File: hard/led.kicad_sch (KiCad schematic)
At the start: 18 parts, among them J1 WS2812B

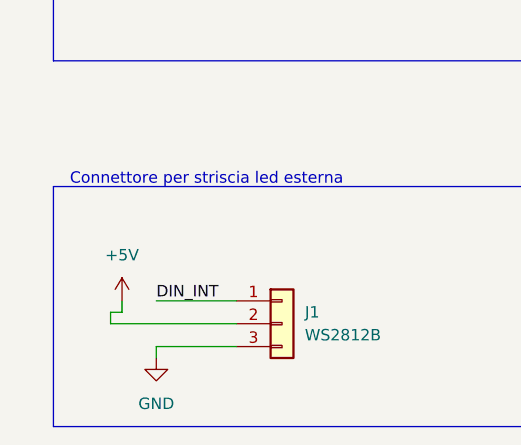
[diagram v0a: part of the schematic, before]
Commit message: update
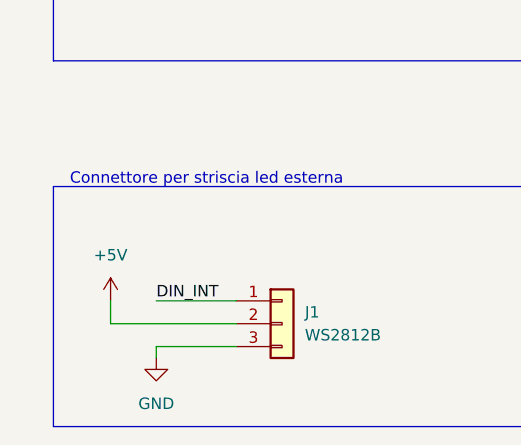
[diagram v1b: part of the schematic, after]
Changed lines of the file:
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@@
-	(wire
-		(pts
-			(xy 21.59 115.57) (xy 22.86 115.57)
-		)
-		(stroke
-			(width 0)
-			(type default)
-		)
-	)
 	(wire
 		(pts
@@
 	(wire
 		(pts
-			(xy 21.59 116.84) (xy 21.59 115.57)
-		)
-		(stroke
-			(width 0)
-			(type default)
-		)
-	)
-	(wire
-		(pts
 			(xy 129.54 39.37) (xy 129.54 50.8)
 		)
@@
 	(wire
 		(pts
-			(xy 22.86 115.57) (xy 22.86 114.3)
+			(xy 21.59 114.3) (xy 21.59 116.84)
 		)
 		(stroke
@@
 	(symbol
 		(lib_id "power:+5V")
-		(at 22.86 114.3 0)
+		(at 21.59 114.3 0)
 		(unit 1)
 		(exclude_from_sim no)
@@
 		(fields_autoplaced yes)
 		(property "Reference" "#PWR099"
-			(at 22.86 118.11 0)
+			(at 21.59 118.11 0)
 			(effects
 				(font
@@
 		)
 		(property "Value" "+5V"
-			(at 22.86 109.22 0)
+			(at 21.59 109.22 0)
 			(effects
 				(font
@@
 		)
 		(property "Footprint" ""
-			(at 22.86 114.3 0)
+			(at 21.59 114.3 0)
 			(effects
 				(font
@@
 		)
 		(property "Datasheet" ""
-			(at 22.86 114.3 0)
+			(at 21.59 114.3 0)
 			(effects
 				(font
@@
 		)
 		(property "Description" "Power symbol creates a global label with name \"+5V\""
-			(at 22.86 114.3 0)
-			(effects
-				(font
+			(at 21.59 114.3 0)
+			(effects
+				(font

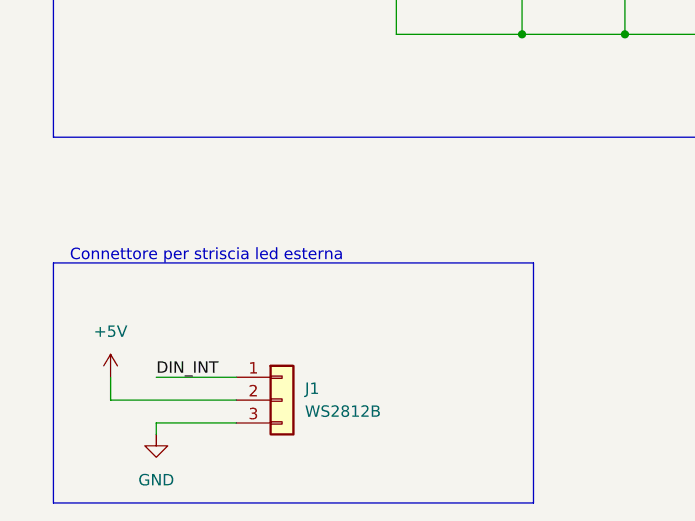
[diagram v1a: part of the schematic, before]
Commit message: update
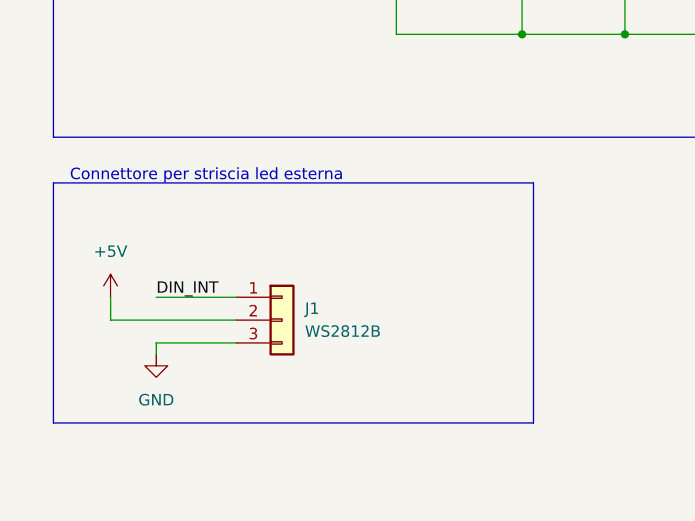
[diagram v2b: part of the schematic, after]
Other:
- title: (none) -> Moduli RGB e LED
- moved on the sheet: J1
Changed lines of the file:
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@@
 	(generator_version "9.0")
 	(paper "A4")
+	(title_block
+		(title "Moduli RGB e LED")
+	)
 	(rectangle
 		(start 15.24 17.78)
@@
 	)
 	(rectangle
-		(start 15.24 101.6)
-		(end 68.58 128.27)
+		(start 15.24 92.71)
+		(end 68.58 119.38)
 		(stroke
 			(width 0)
@@
 	(text "Connettore per striscia led esterna"
 		(exclude_from_sim no)
-		(at 32.258 100.838 0)
+		(at 32.258 91.948 0)
 		(effects
 			(font
@@
 	(wire
 		(pts
-			(xy 26.67 114.3) (xy 35.56 114.3)
+			(xy 26.67 105.41) (xy 35.56 105.41)
 		)
 		(stroke
@@
 	(wire
 		(pts
-			(xy 35.56 119.38) (xy 26.67 119.38)
+			(xy 35.56 110.49) (xy 26.67 110.49)
 		)
 		(stroke
@@
 	(wire
 		(pts
-			(xy 35.56 116.84) (xy 21.59 116.84)
+			(xy 35.56 107.95) (xy 21.59 107.95)
 		)
 		(stroke
@@
 	(wire
 		(pts
-			(xy 26.67 119.38) (xy 26.67 120.65)
+			(xy 26.67 110.49) (xy 26.67 111.76)
 		)
 		(stroke
@@
 	(wire
 		(pts
-			(xy 21.59 114.3) (xy 21.59 116.84)
+			(xy 21.59 105.41) (xy 21.59 107.95)
 		)
 		(stroke
@@
 	)
 	(label "DIN_INT"
-		(at 26.67 114.3 0)
+		(at 26.67 105.41 0)
 		(effects
 			(font
@@
 	(symbol
 		(lib_id "Connector_Generic:Conn_01x03")
-		(at 40.64 116.84 0)
+		(at 40.64 107.95 0)
 		(unit 1)
 		(exclude_from_sim no)
@@
 		(fields_autoplaced yes)
 		(property "Reference" "J1"
-			(at 43.18 115.5699 0)
+			(at 43.18 106.6799 0)
 			(effects
 				(font
@@
 		)
 		(property "Value" "WS2812B"
-			(at 43.18 118.1099 0)
+			(at 43.18 109.2199 0)
 			(effects
 				(font
@@
 		)
 		(property "Footprint" "Connector_PinHeader_2.54mm:PinHeader_1x03_P2.54mm_Vertical"
-			(at 40.64 116.84 0)
+			(at 40.64 107.95 0)
 			(effects
 				(font
@@
 		)
 		(property "Datasheet" "~"
-			(at 40.64 116.84 0)
+			(at 40.64 107.95 0)
 			(effects
 				(font
@@
 		)
 		(property "Description" "Generic connector, single row, 01x03, script generated (kicad-library-utils/schlib/autogen/connector/)"
-			(at 40.64 116.84 0)
+			(at 40.64 107.95 0)
 			(effects
 				(font
@@
 	(symbol
 		(lib_id "power:+5V")
-		(at 21.59 114.3 0)
+		(at 21.59 105.41 0)
 		(unit 1)
 		(exclude_from_sim no)
@@
 		(fields_autoplaced yes)
 		(property "Reference" "#PWR099"
-			(at 21.59 118.11 0)
+			(at 21.59 109.22 0)
 			(effects
 				(font
@@
 		)
 		(property "Value" "+5V"
-			(at 21.59 109.22 0)
+			(at 21.59 100.33 0)
 			(effects
 				(font
@@
 		)
 		(property "Footprint" ""
-			(at 21.59 114.3 0)
+			(at 21.59 105.41 0)
 			(effects
 				(font
@@
 		)
 		(property "Datasheet" ""
-			(at 21.59 114.3 0)
+			(at 21.59 105.41 0)
 			(effects
 				(font
@@
 		)
 		(property "Description" "Power symbol creates a global label with name \"+5V\""
-			(at 21.59 114.3 0)
+			(at 21.59 105.41 0)
 			(effects
 				(font
@@
 	(symbol
 		(lib_id "power:GND")
-		(at 26.67 120.65 0)
+		(at 26.67 111.76 0)
 		(unit 1)
 		(exclude_from_sim no)
@@
 		(fields_autoplaced yes)
 		(property "Reference" "#PWR0100"
-			(at 26.67 127 0)
+			(at 26.67 118.11 0)
 			(effects
 				(font
@@
 		)
 		(property "Value" "GND"
-			(at 26.67 125.73 0)
+			(at 26.67 116.84 0)
 			(effects
 				(font
@@
 		)
 		(property "Footprint" ""
-			(at 26.67 120.65 0)
+			(at 26.67 111.76 0)
 			(effects
 				(font
@@
 		)
 		(property "Datasheet" ""
-			(at 26.67 120.65 0)
+			(at 26.67 111.76 0)
 			(effects
 				(font
@@
 		)
 		(property "Description" "Power symbol creates a global label with name \"GND\" , ground"
-			(at 26.67 120.65 0)
-			(effects
-				(font
+			(at 26.67 111.76 0)
+			(effects
+				(font
